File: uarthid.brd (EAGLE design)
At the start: 160 x 100 mm, 2 parts, among them IC1 FT230XQ, IC2 MEGA8-MI

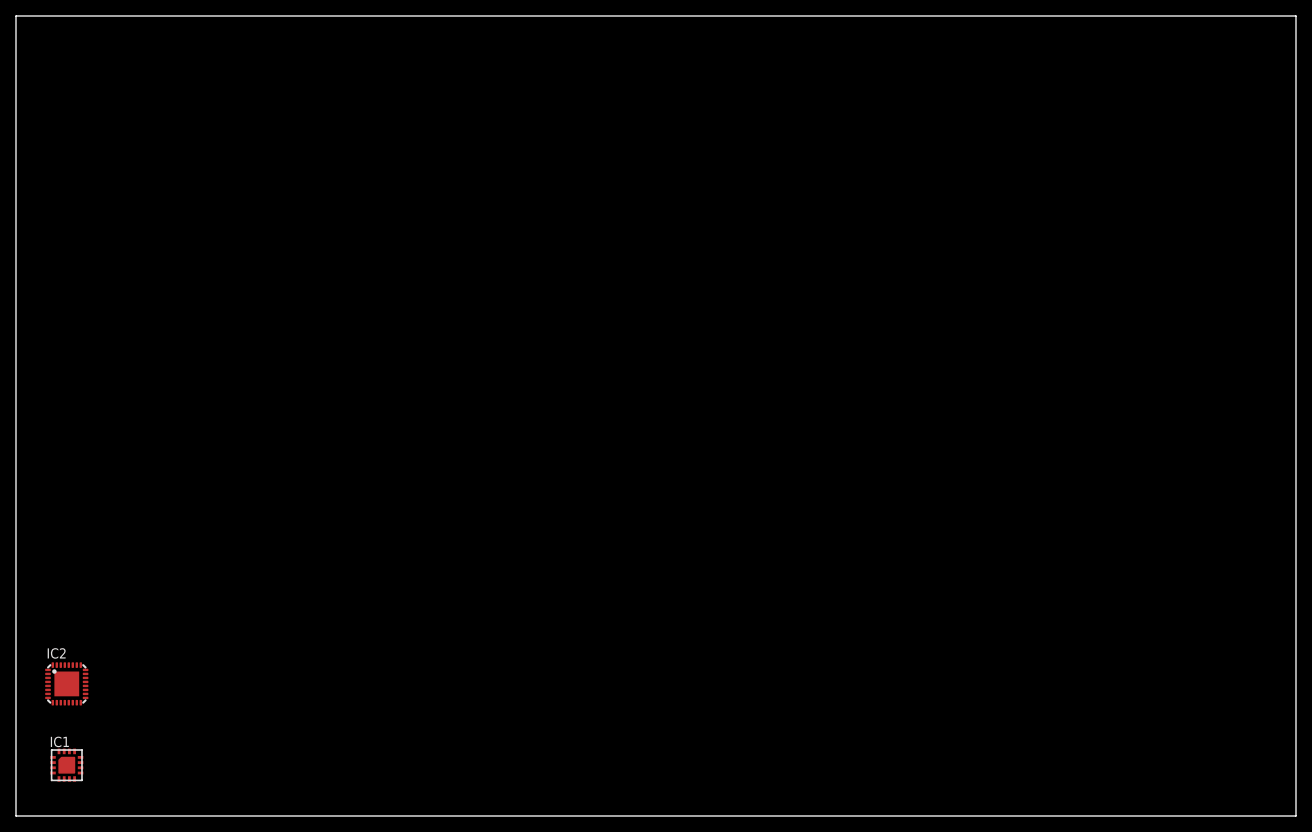
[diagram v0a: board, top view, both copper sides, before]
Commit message: routed and bom'd
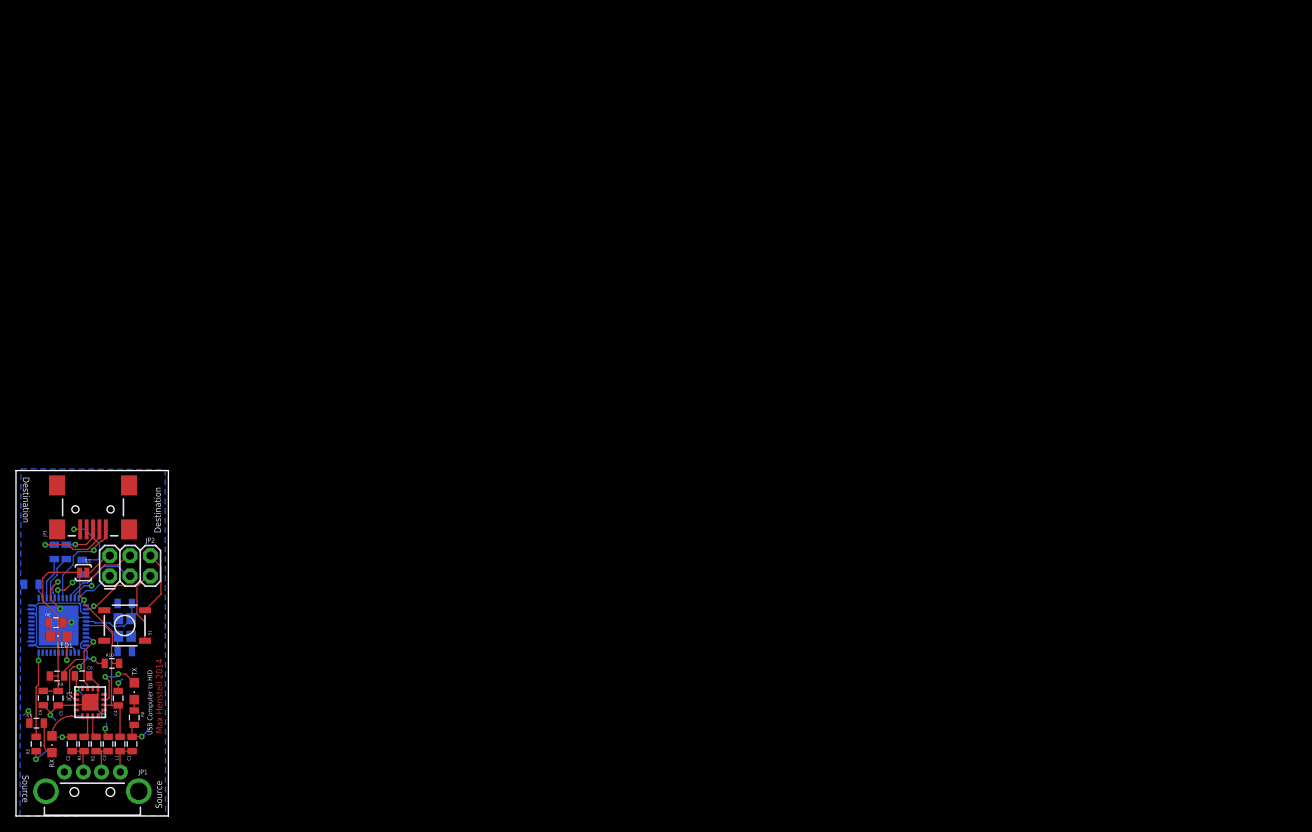
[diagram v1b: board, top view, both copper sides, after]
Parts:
- added C1: 10nF, SparkFun-Capacitors:0805
- added C10, C11: 10pF, SparkFun-Capacitors:0805
- added C2, C3: 47pF, SparkFun-Capacitors:0805
- added C4, C6: 100nF, SparkFun-Capacitors:0805
- added C5: 4.7uF, SparkFun-Capacitors:0805
- added C7: 1uF, SparkFun-Capacitors:0805
- added C8, C9: 0.1uF, SparkFun-Capacitors:0805
- added JP1: USB-A-H, SparkFun-Connectors:USB-A-H
- added JP2: (no value), SparkFun-Connectors:2X3
- added JP3: USBSMD, SparkFun-Connectors:USB-MINIB
- added L1: FERRITE, Livestream:0805
- added LED1, RX, TX: (no value), adafruit:CHIPLED_0805
- added Q1: 16 Mhz, adafruit:NX3225
- added R1, R2: 27R, SparkFun-Passives:0805
- added R10, R9: 10k, SparkFun-Passives:0805
- added R3, R4: 22, SparkFun-Passives:0805
- added R5, R6: 1k, SparkFun-Passives:0805
- added R7, R8: 270, SparkFun-Passives:0805
- added S1: (no value), SparkFun-Electromechanical:TACTILE_SWITCH_SMD
- added SJ1: SOLDERJUMPERNO, SparkFun-Passives:SJ_2S-NO
- IC2: value MEGA8-MI -> 32u4; device avr-5:MLF32 -> SparkFun-DigitalIC:SPARKFUN-DIGITALIC_QFN-44
- moved IC1 8.40 mm to (9.27, 14.2)
- moved IC2 7.38 mm to (5.33, 23.8), flipped to the bottom, turned to 270 degrees
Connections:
- removed net VCCIO: IC1.1
- new net 3V3OUT: C6.1, IC1.1, IC1.8, IC1.9
- new net FT_RX: IC1.2, IC2.21, R10.1
- new net FT_TX: IC1.15, IC2.20, R9.1
- new net N$1: C2.1, JP1.D+, R1.1
- new net N$10: JP2.2, SJ1.1
- new net N$11: C7.1, IC2.6
- new net N$12: IC2.11, JP2.1
- new net N$13: IC2.9, JP2.3
- new net N$14: IC2.10, JP2.4
- new net N$15: IC2.33, R5.2
- new net N$16: IC2.26, LED1.A
- new net N$17: LED1.C, R6.2
- new net N$18: IC1.11, TX.A
- new net N$19: R7.1, RX.C
- new net N$2: IC1.6, R1.2
- new net N$20: R8.1, TX.C
- new net N$3: C3.1, JP1.D-, R2.1
- new net N$4: IC1.7, R2.2
- new net N$5: C1.1, JP1.VBUS, L1.1
- new net N$6: C10.2, IC2.17, Q1.1
- new net N$7: C11.2, IC2.16, Q1.3
- new net N$8: JP3.D-, R3.2
- new net N$9: JP3.D+, R4.2
- new net RST: IC2.13, JP2.5, S1.1
- new net RX_LED: IC1.5, RX.A
- new net USB_DM: IC2.3, R3.1
- new net USB_DP: IC2.4, R4.1
- new net USB_VBUS: IC2.7, JP3.VBUS
- net GND: now also C1.2, C10.1, C11.1, C2.2, C3.2, C4.2, C5.2, C6.2, C7.2, C8.2, C9.2, IC1.TAB, IC2.15, IC2.23, IC2.35, IC2.43, IC2.5, JP1.GND, JP2.6, JP3.GND, Q1.2, Q1.4, R5.1, R6.1, R7.2, R8.2, S1.3
- net VCC: now also C4.1, C5.1, C8.1, C9.1, IC2.14, IC2.2, IC2.24, IC2.34, IC2.42, IC2.44, L1.2, R10.2, R9.2, SJ1.2
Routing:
- net VCC: track 0.00 -> 71.0 mm, vias 0 -> 1
- net GND: track 0.00 -> 60.5 mm, vias 0 -> 11
- net RST: track 0.00 -> 17.1 mm, vias 0 -> 1
- net FT_RX: track 0.00 -> 12.6 mm, vias 0 -> 2
- net USB_VBUS: track 0.00 -> 12.0 mm, vias 0 -> 1
- net FT_TX: track 0.00 -> 11.4 mm, vias 0 -> 1
- net N$15: track 0.00 -> 10.7 mm, vias 0 -> 1
- net N$14: track 0.00 -> 9.90 mm, vias 0 -> 1
- net N$13: track 0.00 -> 9.84 mm
- net N$8: track 0.00 -> 9.79 mm, vias 0 -> 1
- net 3V3OUT: track 0.00 -> 8.73 mm, vias 0 -> 2
- net N$7: track 0.00 -> 8.29 mm
- net N$18: track 0.00 -> 7.76 mm, vias 0 -> 2
- net N$6: track 0.00 -> 6.59 mm
- net USB_DP: track 0.00 -> 5.74 mm
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- added copper zone on layer 16, net GND
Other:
- board size 160 x 100 mm -> 19.1 x 43.2 mm
- board text added: "Destination"
- board text added: "Max Henstell 2014"
- board text added: "Source"
- board text added: "USB Computer to HID"
